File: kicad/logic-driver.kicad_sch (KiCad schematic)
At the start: 27 parts, among them J1 TIMEPULSE, J2 TIMEPULSE2, J3 LCD signal, J4 LCD GND, J5 LCD bias, J6 LCD bias, U3 4011, U4 4070, U5 4013, U6 TL074

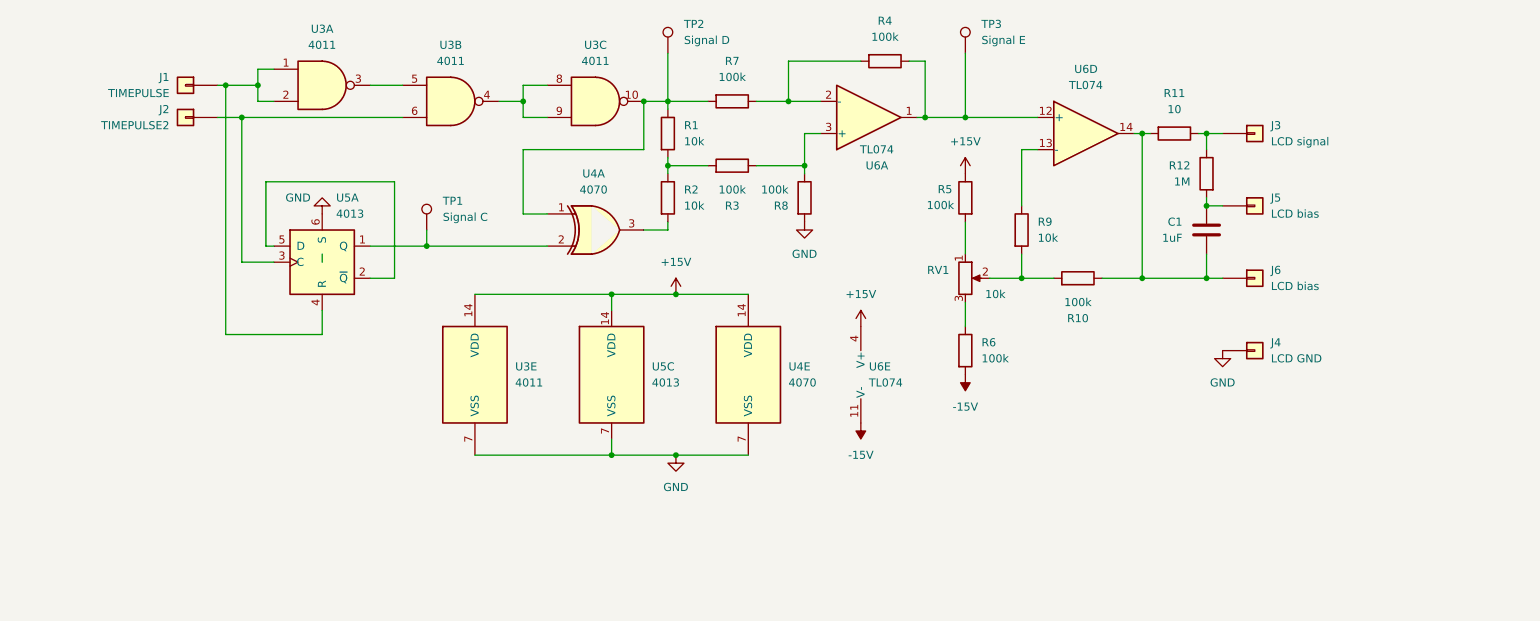
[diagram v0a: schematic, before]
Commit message: Updates the electronic schema
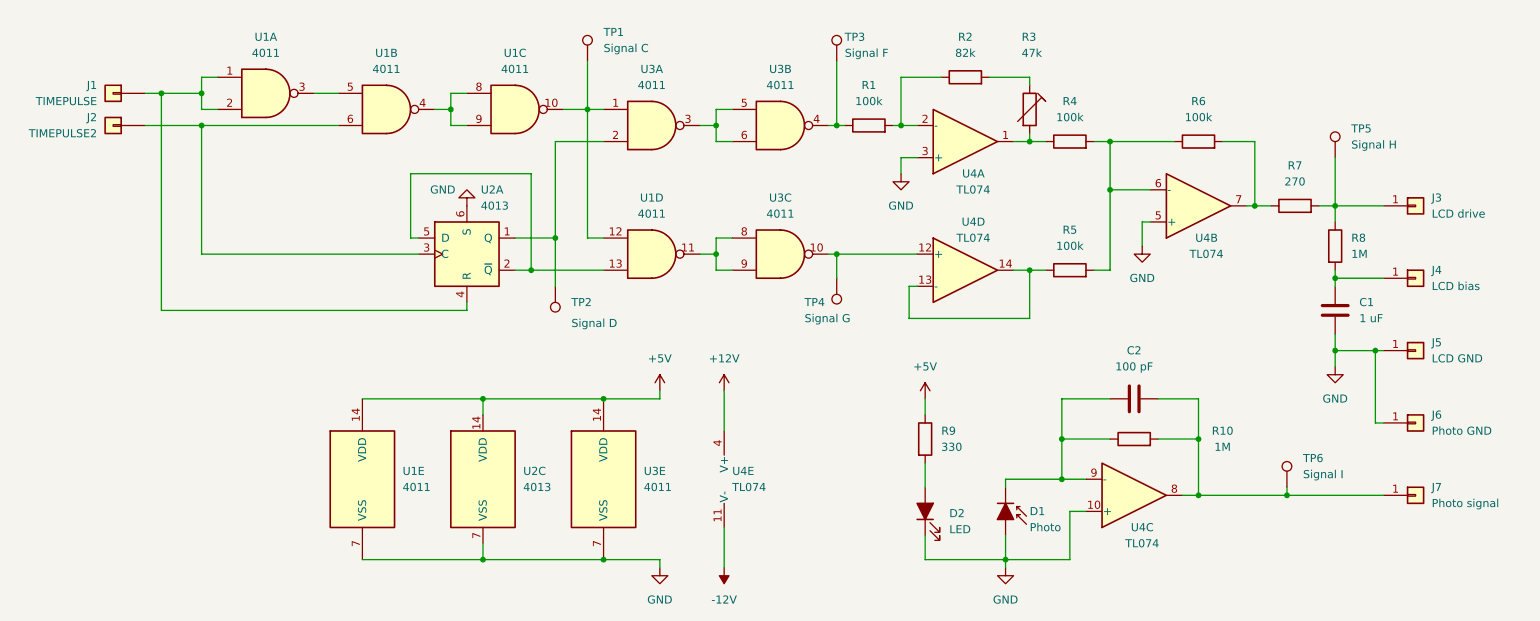
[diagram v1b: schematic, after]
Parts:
- removed R11: 10, symbol Device:R
- removed R12: 1M, symbol Device:R
- removed R3: 100k, symbol Device:R
- removed RV1: 10k, symbol Device:R_Potentiometer
- removed U4: 4070, symbol 4xxx:4070
- removed U5: 4013, symbol 4xxx:4013
- removed U6: TL074, symbol Amplifier_Operational:TL074
- added C2: 100 pF, symbol Device:C
- added D1: Photo, symbol Device:D_Photo_Filled
- added D2: LED, symbol Device:LED_Filled
- added J7: Photo signal, symbol Connector_Generic:Conn_01x01
- added R3: 47k, symbol Device:R_Trim
- added TP4: Signal G, symbol Connector:TestPoint
- added TP5: Signal H, symbol Connector:TestPoint
- added TP6: Signal I, symbol Connector:TestPoint
- added U1: 4011, symbol 4xxx:4011
- added U2: 4013, symbol 4xxx:4013
- added U4: TL074, symbol Amplifier_Operational:TL074
- C1: value 1uF -> 1 uF
- J3: value LCD signal -> LCD drive
- J4: value LCD GND -> LCD bias
- J5: value LCD bias -> LCD GND
- J6: value LCD bias -> Photo GND
- R1: value 10k -> 100k
- R10, R8: value 100k -> 1M
- R2: value 10k -> 82k
- R7: value 100k -> 270
- R9: value 10k -> 330
- TP3: value Signal E -> Signal F
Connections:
- net GND: now also C1.2, J5.1 (Pin_1), J6.1 (Pin_1), D1.2 (A), D2.1 (K), U1.7 (VSS), U2.6 (S), U2.7 (VSS), U4.10 (+), U4.3 (+), U4.5 (+); no longer J4.1 (Pin_1), R8.2
- net at U3.8, U3.9: now also U1.11; no longer U3.4
- net at TP1.1: now also U3.1, U1.10, U1.12
- net at J2.1 (Pin_1): now also U1.6, U2.3 (C); no longer U3.6
- net at U3.3, U3.5: now also U3.6
- net at R1.2, R2.1: now also U4.2 (-)
- net at R2.2: now also R3.1
- net at TP3.1: now also R1.1, U3.4; no longer R4.1
- net at R4.2: now also R5.2, R6.1, U4.6 (-); no longer R7.1
- net at R8.1: now also J3.1 (Pin_1), R7.2, TP5.1
- net at R9.2: now also D2.2 (A); no longer R10.2
- net +5V: now reaches R9.1
- net +5V: now also U3.14 (VDD), U1.14 (VDD), U2.14 (VDD)
- net at C1.1: now also J4.1 (Pin_1), R8.2; no longer J5.1 (Pin_1)
- net +15V: no longer names the net of R5.1
- net +15V: now also U4.13 (-), U4.14; no longer U3.14 (VDD)
- net -15V: no longer names the net of R6.2
- net -15V: now also R7.1, U4.7
- new net: U1.13, U2.2 (~{Q}), U2.5 (D)
- new net: TP4.1, U3.10, U4.12 (+)
- new net: J1.1 (Pin_1), U1.1, U1.2, U2.4 (R)
- new net: C2.2, J7.1 (Pin_1), R10.2, TP6.1, U4.8
- new net: R3.2, R4.1, U4.1
- new net: U1.4, U1.8, U1.9
- new net: U1.3, U1.5
- new net: C2.1, D1.1 (K), R10.1, U4.9 (-)
- new net: TP2.1, U2.1 (Q), U3.2
- new net +12V: U4.4 (V+)
- new net -12V: U4.11 (V-)
